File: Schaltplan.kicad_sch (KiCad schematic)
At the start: 16 parts, among them K1 Relay, P1 USB Port vorheriger, P2 USB Port nächster, P4 USB Port Laden, U1 DC DC Wandler, U2 DC DC Wandler, U3 Digitaler Poti, U4 Display, U5 DC DC Wandler, U6 Digitaler Poti, U8 Amperemeter, U9 DS18B20

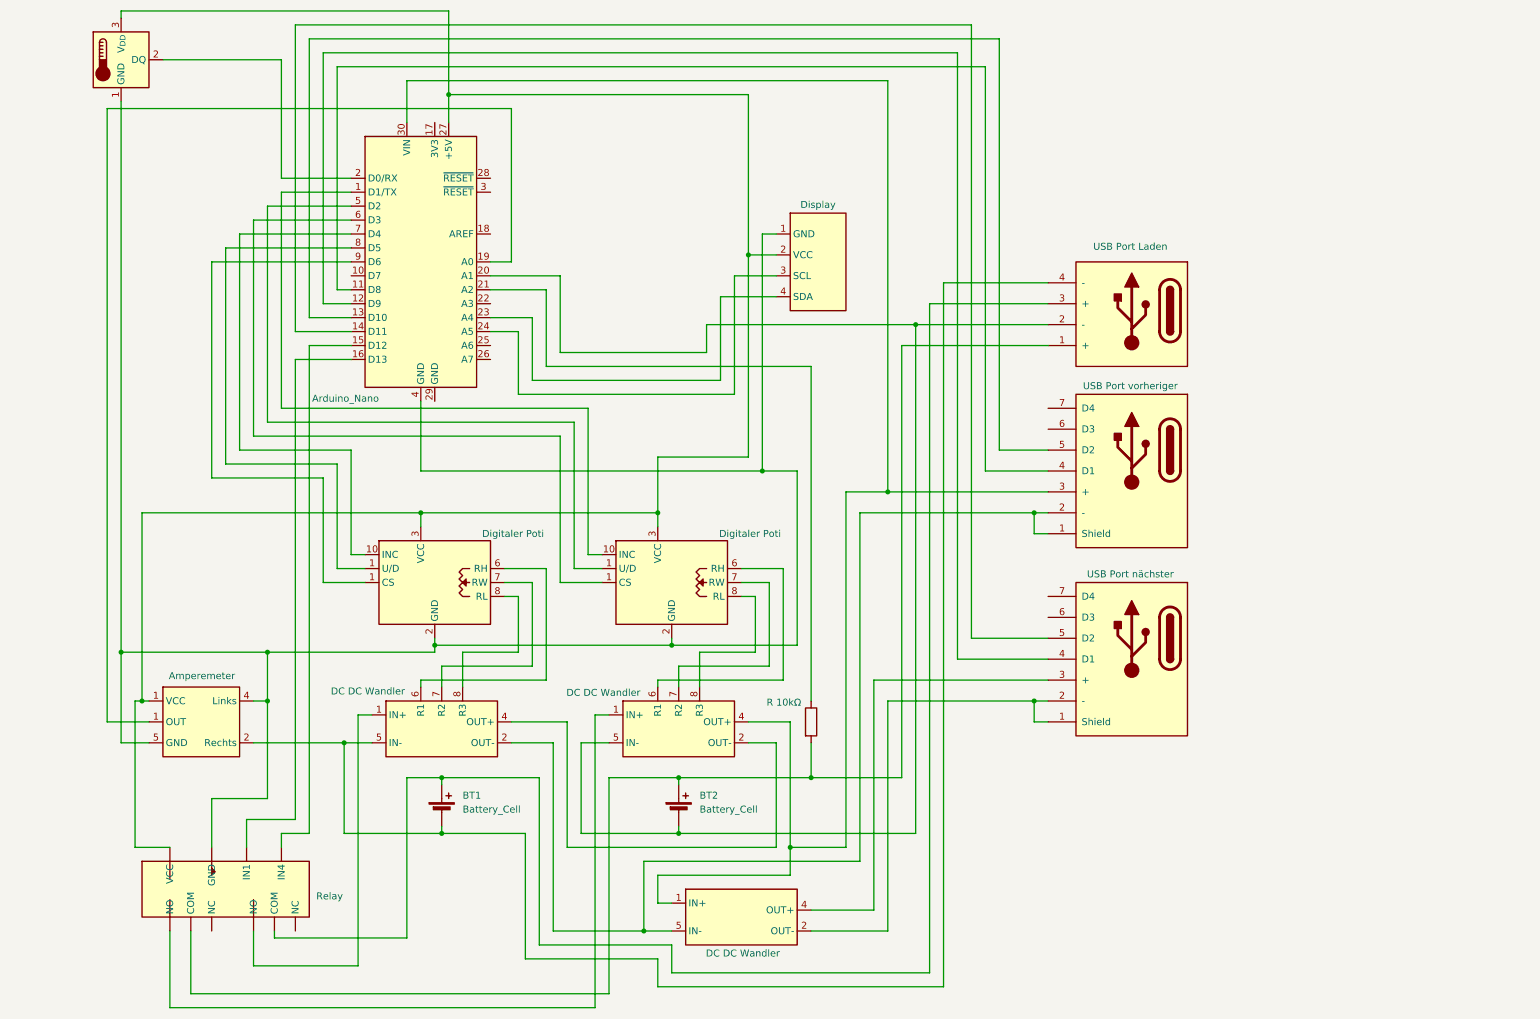
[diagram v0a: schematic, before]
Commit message: Commit
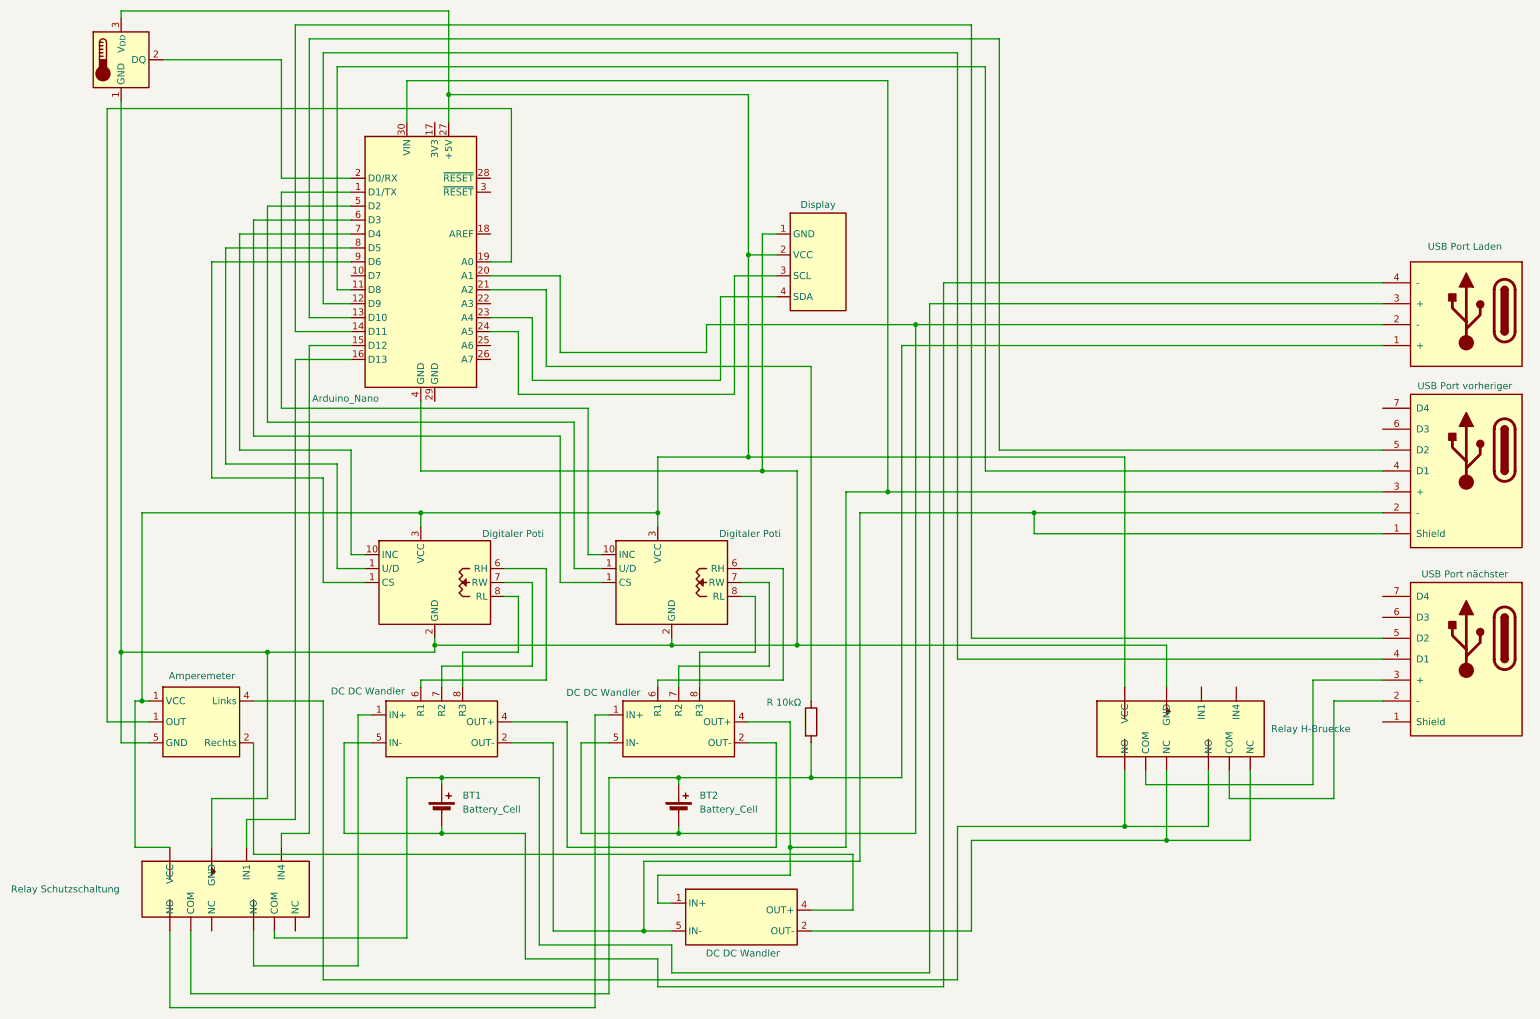
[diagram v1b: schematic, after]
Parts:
- added K2: Relay H-Bruecke, symbol Relay:Relay_DPST-NC
- K1: value Relay -> Relay Schutzschaltung
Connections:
- net at BT1.2 (-), P4.4 (-), U2.5 (IN-): no longer U8.2 (Rechts)
- net at A1.4 (GND), K1. (NC), U3.2 (GND)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: now also K2. (NC); no longer U8.4 (Links)
- net at A1.27 (+5V), K1. (NC), U3.3 (VCC)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: now also K2. (NC)
- net at P2.3 (+): now also K2. (NC); no longer U5.4 (OUT+)
- net at K1. (NC): now also A1.16 (D13)
- new net: K2. (NC), U5.2 (OUT-)
- new net: K2. (NC), P2.2 (-)
- new net: K2. (NC), U8.4 (Links)
- new net: U5.4 (OUT+), U8.2 (Rechts)
- now unconnected: P2.1 (Shield)
